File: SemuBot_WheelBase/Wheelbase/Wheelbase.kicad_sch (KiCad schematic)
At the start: 60 parts, among them J1 10155435-00011LF, J10 B5B-XH-A_LF__SN_, J11 B5B-XH-A_LF__SN_, J12 B5B-XH-A_LF__SN_, J13 MTSW-104-09-L-S-400, J14 XT30PW-M, J3 MR30PW-M, J4 B5B-XH-A_LF__SN_, J5 B5B-XH-A_LF__SN_, J6 B5B-XH-A_LF__SN_, J7 MR30PW-M, J8 MR30PW-M, J9 DS1013-10SSIB1, U1 STM32G474RET6, U5 RT9013-33GB, Y2 X322516MLB4SI

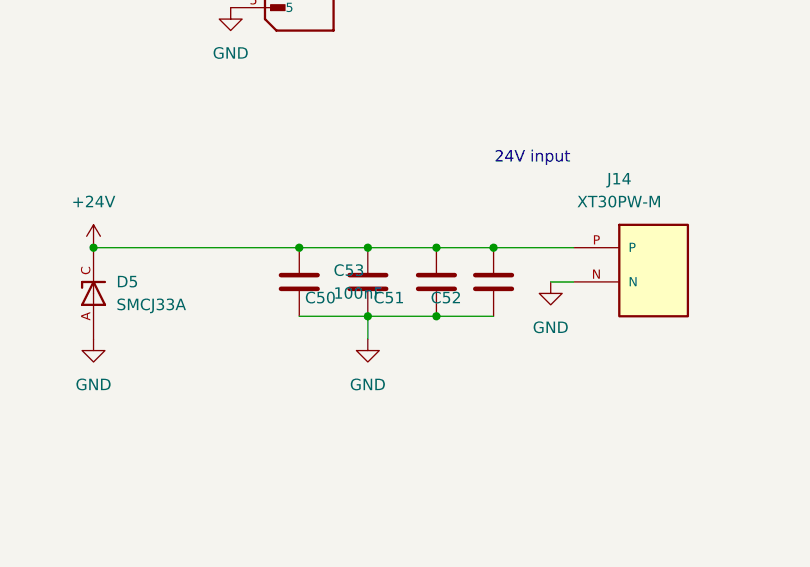
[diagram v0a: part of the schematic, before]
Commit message: Schematic and pcb fix
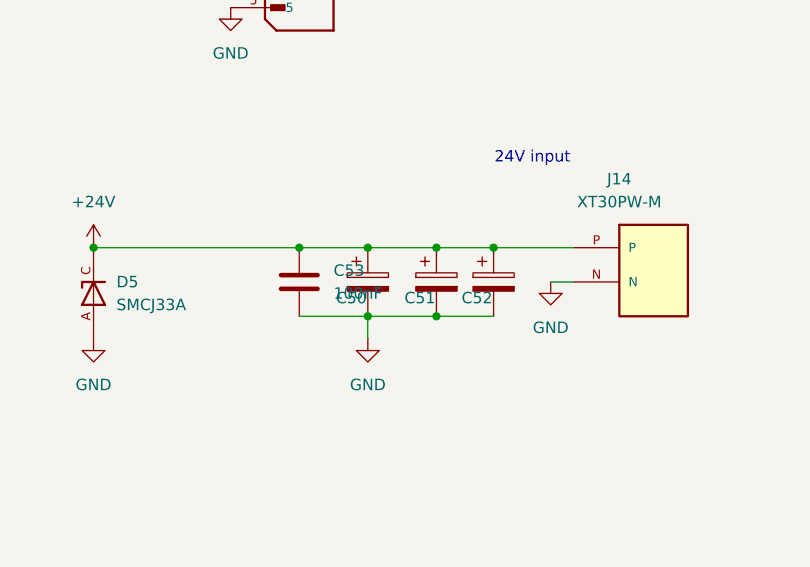
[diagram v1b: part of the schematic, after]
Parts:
- C50, C51, C52: symbol Device:C -> Device:C_Polarized
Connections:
- net +24V: now also C50.1, C51.1, C52.1; no longer C50.2, C51.2, C52.2
- net GND: now also C50.2, C51.2, C52.2; no longer C50.1, C51.1, C52.1
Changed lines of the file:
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@@
 	)
 	(symbol
-		(lib_id "Device:C")
-		(at 322.58 171.45 180)
+		(lib_id "Device:C_Polarized")
+		(at 322.58 171.45 0)
 		(unit 1)
 		(body_style 1)
@@
 	)
 	(symbol
-		(lib_id "Device:C")
-		(at 328.93 171.45 180)
+		(lib_id "Device:C_Polarized")
+		(at 328.93 171.45 0)
 		(unit 1)
 		(body_style 1)
@@
 	)
 	(symbol
-		(lib_id "Device:C")
-		(at 314.96 171.45 180)
+		(lib_id "Device:C_Polarized")
+		(at 314.96 171.45 0)
 		(unit 1)
 		(body_style 1)
